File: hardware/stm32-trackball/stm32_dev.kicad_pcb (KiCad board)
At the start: 2 copper layers, 80.8 x 30 mm, 60 parts, among them J1 USB_C_Receptacle_USB2.0, J2 SWD, J3 UART, J4 SPARE, J5 Breakout, J6 Breakout, SW1 KMR2, SW2 KMR2, SW3 SW_Push, SW4 KMR2, SW5 KMR2, SW6 KMR2, T1 Trackball, U1 AP2112K-3.3, U2 USBLC6-2SC6, U3 STM32F042G6Ux, U4 AN48840B, U5 AN48840B, U6 AN48840B, U7 AN48840B

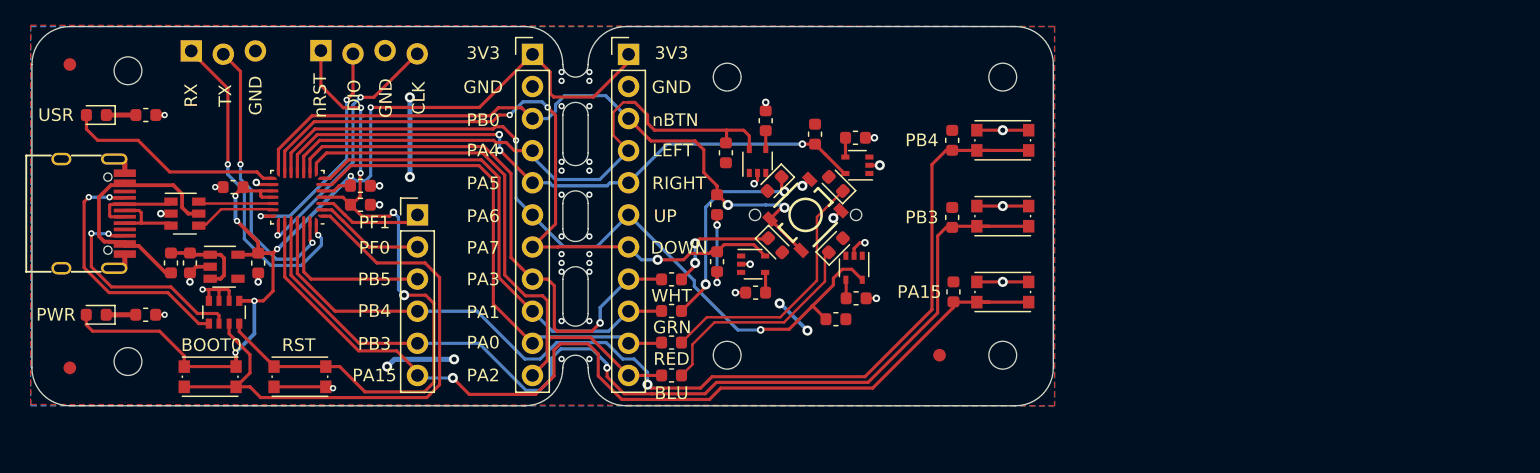
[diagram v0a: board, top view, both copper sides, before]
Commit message: 2u layout somehow passes DRC
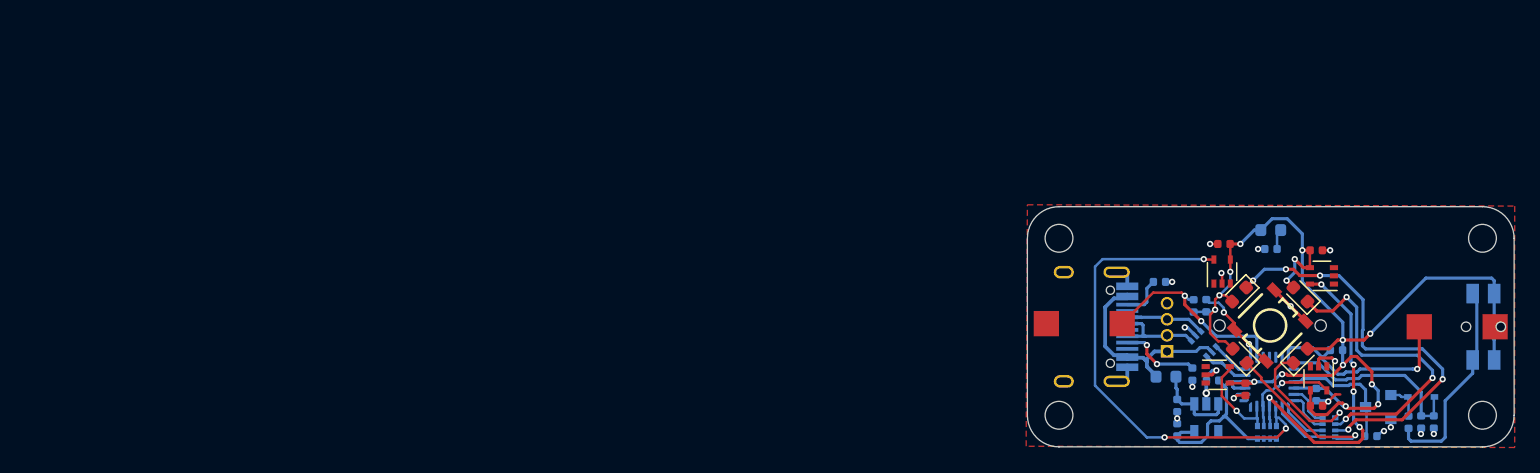
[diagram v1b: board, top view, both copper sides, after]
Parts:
- removed C2: 100n, Capacitor_SMD:C_0603_1608Metric
- removed D1: LED, LED_SMD:LED_0603_1608Metric
- removed H1, H2, H3: Fuduical, Fiducial:Fiducial_1mm_Mask2mm
- removed H8, H9: M2, MountingHole:MountingHole_2.2mm_M2
- removed J3: UART, josh-connectors:STM_3_PIN_THT_Staggered
- removed J4: SPARE, Connector_PinHeader_2.54mm:PinHeader_1x06_P2.54mm_Vertical
- removed J5, J6: Breakout, Connector_PinHeader_2.54mm:PinHeader_1x11_P2.54mm_Vertical
- removed R10, R7, R8, R9: 220R, Resistor_SMD:R_0603_1608Metric
- removed R5, R6: 10K, Resistor_SMD:R_0603_1608Metric
- removed SW5, SW6: KMR2, josh-buttons-switches:SW_Push_KMR2
- added C11: 10u, Capacitor_SMD:C_0402_1005Metric, B.Cu at (179.9, 117.3)
- added C12: 4u7, Capacitor_SMD:C_0402_1005Metric, B.Cu at (175.9, 118.4)
- added D7: 1N4148, Diode_SMD:D_SOD-323, B.Cu at (179.9, 115.3)
- added Q3: DTC123J, Package_TO_SOT_SMD:SOT-23, B.Cu at (176.5, 116.1)
- added RN2: 2K2, Resistor_SMD:R_Array_Convex_4x0402, B.Cu at (172.6, 117.7)
- C1, C3, C5, C6: footprint Capacitor_SMD:C_0603_1608Metric -> Capacitor_SMD:C_0402_1005Metric; moved to B.Cu
- C10, C7, C8, C9: footprint Capacitor_SMD:C_0603_1608Metric -> Capacitor_SMD:C_0402_1005Metric
- D2, F1, J1, U1, U3: moved to B.Cu
- J2: value SWD -> USB; footprint josh-connectors:STM_4_PIN_THT_Staggered -> Connector_PinHeader_1.27mm:PinHeader_1x04_P1.27mm_Vertical; moved to B.Cu
- R1: value 2K2 -> 5K1; footprint Resistor_SMD:R_0603_1608Metric -> Resistor_SMD:R_0402_1005Metric; moved to B.Cu
- R11, R12, R2, R4: footprint Resistor_SMD:R_0603_1608Metric -> Resistor_SMD:R_0402_1005Metric; moved to B.Cu
- R13: value 10K -> 2K2; footprint Resistor_SMD:R_0603_1608Metric -> Resistor_SMD:R_0402_1005Metric; moved to B.Cu
- R14: value 10K -> 100K; footprint Resistor_SMD:R_0603_1608Metric -> Resistor_SMD:R_0402_1005Metric; moved to B.Cu
- R3: value 10K -> 5K1; footprint Resistor_SMD:R_0603_1608Metric -> Resistor_SMD:R_0402_1005Metric; moved to B.Cu
- RN1: value 5K1 -> 10K; footprint Resistor_SMD:R_Array_Convex_4x0603 -> Resistor_SMD:R_Array_Convex_4x0402; moved to B.Cu
- SW1: value KMR2 -> SW_Push; footprint josh-buttons-switches:SW_Push_KMR2 -> josh-buttons-switches:Panasonic_EVQPUL_EVQPUC; moved to B.Cu
- SW2, SW4: value KMR2 -> BIG; footprint josh-buttons-switches:SW_Push_KMR2 -> josh-buttons-switches:Switch_SMT_SKPMAPE010
- U2: footprint Package_TO_SOT_SMD:SOT-23-6 -> Package_TO_SOT_SMD:SOT-666; moved to B.Cu
- moved H5 107.6 mm to (184.8, 102.8)
- moved SW1 100.8 mm to (184.8, 109.8), turned to 90 degrees
- moved SW2 94.6 mm to (185.8, 109.8)
- moved D2 93.2 mm to (168.0, 102.1)
- moved R2 89.2 mm to (168.0, 103.6), turned to 180 degrees
- moved R1 85.3 mm to (161.8, 113.5), turned to 90 degrees
- moved RN1 83.0 mm to (167.7, 118.1)
- moved U2 81.3 mm to (162.7, 111.1), turned to 315 degrees
- moved J1 79.8 mm to (153.5, 109.8), turned to 90 degrees
- moved F1 79.2 mm to (159.7, 113.7), turned to 180 degrees
- moved C5 79.0 mm to (163.4, 114.0)
- moved C1 78.9 mm to (160.6, 116.0)
- moved U1 78.6 mm to (162.9, 117.0), turned to 270 degrees
- moved H6 78.5 mm to (151.2, 116.8)
- moved U3 78.3 mm to (167.9, 114.1)
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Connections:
- C1 pad 2: VBUS -> +5V
- F1 pad 1: VBUS -> +5V
- F1 pad 2: Net-(F1-Pad2) -> VBUS
- J1 pad A4: Net-(F1-Pad2) -> VBUS
- J1 pad A9: Net-(F1-Pad2) -> VBUS
- J1 pad B4: Net-(F1-Pad2) -> VBUS
- J1 pad B9: Net-(F1-Pad2) -> VBUS
- J2 pad 1: /nRST -> VBUS
- J2 pad 2: /SWDIO -> /USB-
- J2 pad 3: GND -> /USB+
- J2 pad 4: /SWDCLK -> GND
- R1 pad 1: Net-(D1-Pad1) -> GND
- R1 pad 2: GND -> Net-(J1-PadA5)
- R12 pad 2: /SPARE_4 -> /BTN_L
- R13 pad 1: +3V3 -> Net-(D7-Pad2)
- R13 pad 2: /SPARE_5 -> Net-(R13-Pad2)
- R14 pad 1: +3V3 -> /BOOT0
- R14 pad 2: /SPARE_6 -> GND
- R3 pad 1: +3V3 -> GND
- R3 pad 2: /TB_LEFT -> Net-(J1-PadB5)
- R4 pad 2: /TB_RIGHT -> /BTN_R
- RN1 pad 1: +3V3 -> /TB_DOWN
- RN1 pad 2: GND -> /TB_RIGHT
- RN1 pad 3: GND -> /TB_UP
- RN1 pad 4: GND -> /TB_LEFT
- RN1 pad 5: Net-(J1-PadA5) -> +3V3
- RN1 pad 6: Net-(J1-PadB5) -> +3V3
- RN1 pad 7: /BOOT0 -> +3V3
- RN1 pad 8: /nRST -> +3V3
- SW1 pad 1: /BOOT0 -> +3V3
- SW1 pad 2: +3V3 -> Net-(R13-Pad2)
- SW2 pad 2: /nRST -> /BTN_R
- SW4 pad 2: /SPARE_4 -> /BTN_L
- U1 pad 1: VBUS -> +5V
- U1 pad 3: VBUS -> +5V
- U2 pad 5: Net-(F1-Pad2) -> VBUS
- U3 pad 14: /nTB_BUTTON -> (no net)
- U3 pad 15: /USR_LED -> (no net)
- U3 pad 2: /SPARE_2 -> (no net)
- U3 pad 21: /SWDIO -> (no net)
- U3 pad 22: /SWDCLK -> /nTB_BUTTON
- U3 pad 23: /SPARE_6 -> /BTN_L
- U3 pad 24: /SPARE_5 -> (no net)
- U3 pad 25: /SPARE_4 -> (no net)
- U3 pad 26: /SPARE_3 -> (no net)
- U3 pad 27: /UART_TX -> (no net)
- U3 pad 28: /UART_RX -> /BTN_R
- U3 pad 3: /SPARE_1 -> (no net)
- U3 pad 6: /nLED_RED -> /nLED_BLU
- U3 pad 7: /nLED_GRN -> /nLED_RED
- U3 pad 8: /nLED_BLU -> /nLED_GRN
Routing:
- net /SPARE_4: track 82.9 -> 0.00 mm, vias 1 -> 0
- net /SPARE_5: track 81.1 -> 0.00 mm, vias 1 -> 0
- net /SPARE_6: track 77.5 -> 0.00 mm, vias 1 -> 0
- net /TB_RIGHT: track 63.8 -> 8.33 mm, vias 2 -> 1
- net /TB_DOWN: track 56.5 -> 7.73 mm, vias 3 -> 1
- net /nTB_BUTTON: track 55.4 -> 8.27 mm
- net /nRST: track 55.2 -> 9.97 mm, vias 4 -> 0
- net /nLED_BLU: track 46.4 -> 3.50 mm
- net /nLED_WHT: track 43.6 -> 4.55 mm, vias 1 -> 0
- net /nLED_RED: track 39.3 -> 3.44 mm
- net /nLED_GRN: track 38.1 -> 3.70 mm
- net /BOOT0: track 46.9 -> 15.7 mm
- net /UART_RX: track 26.2 -> 0.00 mm, vias 2 -> 0
- net /TB_UP: track 50.2 -> 25.7 mm, vias 3 -> 5
- net /UART_TX: track 23.1 -> 0.00 mm, vias 2 -> 0
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- added copper zone on F.Cu, net GND
- removed copper zone on F.Cu, net +3V3
- removed copper zone on B.Cu, net GND
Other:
- board size 80.8 x 30 mm -> 38.5 x 19 mm
- rule pad_to_mask_clearance: 0.05 -> 0
- rule via_min_drill: 0.3 -> 0.25
- rule via_min_size: 0.4 -> 0.5
- board text removed: "3V3"
- board text removed: "BLU"
- board text removed: "BOOT0"
- board text removed: "CLK"
- board text removed: "DIO"
- board text removed: "DOWN"
- board text removed: "GND"
- board text removed: "GRN"
- board text removed: "LEFT"
- board text removed: "PA0"
- board text removed: "PA1"
- board text removed: "PA15"
- board text removed: "PA2"
- board text removed: "PA3"
- board text removed: "PA4"
- board text removed: "PA5"
- board text removed: "PA6"
- board text removed: "PA7"
- board text removed: "PB0"
- board text removed: "PB3"
- board text removed: "PB4"
- board text removed: "PB5"
- board text removed: "PF0"
- board text removed: "PF1"
- board text removed: "PWR"
- board text removed: "RED"
- board text removed: "RIGHT"
- board text removed: "RST"
- board text removed: "RX"
- board text removed: "TX"
- board text removed: "UP"
- board text removed: "USR"
- board text removed: "WHT"
- board text removed: "nBTN"
- board text removed: "nRST"
